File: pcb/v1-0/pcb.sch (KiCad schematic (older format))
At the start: 0 parts

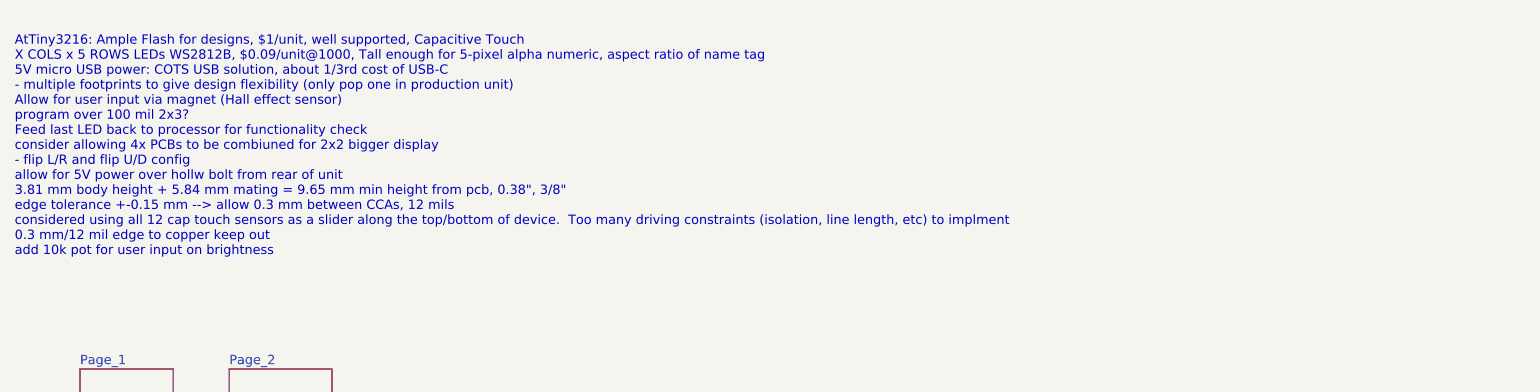
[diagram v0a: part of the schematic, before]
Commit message: compontnets placedr
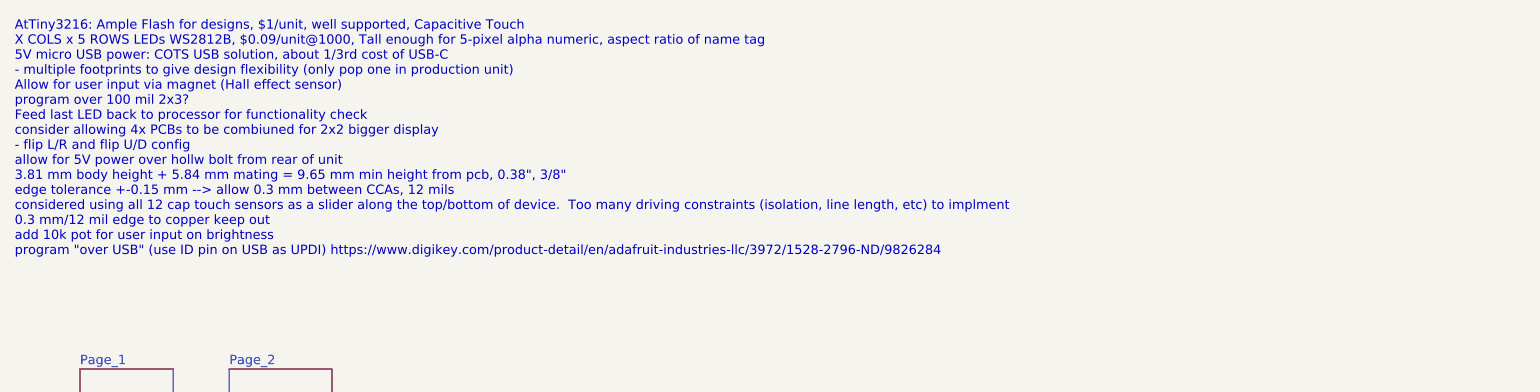
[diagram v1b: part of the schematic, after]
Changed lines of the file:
@@
 verify ws2182 footprint\nverify pinout of led\nwriteup parts list\nattiny: PTC, program, hall effect, USB power, Array led\n2x3 pin #s? conn_02x03\nallow for pogo programming\nensure LEDs are OFF during program upload\nadd UPDI pinout to silk screen\npick screw size, figure out PCB outline\nenter in space between traces into layout preferences\nbuy anodized aluminum\nbuy two color acrylic - info badge\nnameplate screws: threaded standoff caps\ndesign for enclosure - height from LEDs\ntwo-piece standoff panel-hanging brackets\ncaptive pins appear cheaper\nPlastic-Head Thumb Screws\n4-40, 0.33/screw: https://www.mcmaster.com/91185A233/\nusb port on reverse side? no - top side reflow only\nround corners of pcb\nput arrow on RxD and TxD showing data flow direciton\nSense Line thickness should be between 0.1mm to 0.5mm\n T: front panel thickness, 1.6 mm\n6" max line length on sense lines\nmcmaster: metal part to melt into plastic the rigidly hold screw - ref tail from hackaday
 Text Notes 550  1750 0    50   ~ 0
-AtTiny3216: Ample Flash for designs, $1/unit, well supported, Capacitive Touch\nX COLS x 5 ROWS LEDs WS2812B, $0.09/unit@1000, Tall enough for 5-pixel alpha numeric, aspect ratio of name tag\n5V micro USB power: COTS USB solution, about 1/3rd cost of USB-C\n- multiple footprints to give design flexibility (only pop one in production unit)\nAllow for user input via magnet (Hall effect sensor)\nprogram over 100 mil 2x3?\nFeed last LED back to processor for functionality check\nconsider allowing 4x PCBs to be combiuned for 2x2 bigger display\n- flip L/R and flip U/D config\nallow for 5V power over hollw bolt from rear of unit\n3.81 mm body height + 5.84 mm mating = 9.65 mm min height from pcb, 0.38", 3/8"\nedge tolerance +-0.15 mm --> allow 0.3 mm between CCAs, 12 mils\nconsidered using all 12 cap touch sensors as a slider along the top/bottom of device.  Too many driving constraints (isolation, line length, etc) to implment\n0.3 mm/12 mil edge to copper keep out\nadd 10k pot for user input on brightness
+AtTiny3216: Ample Flash for designs, $1/unit, well supported, Capacitive Touch\nX COLS x 5 ROWS LEDs WS2812B, $0.09/unit@1000, Tall enough for 5-pixel alpha numeric, aspect ratio of name tag\n5V micro USB power: COTS USB solution, about 1/3rd cost of USB-C\n- multiple footprints to give design flexibility (only pop one in production unit)\nAllow for user input via magnet (Hall effect sensor)\nprogram over 100 mil 2x3?\nFeed last LED back to processor for functionality check\nconsider allowing 4x PCBs to be combiuned for 2x2 bigger display\n- flip L/R and flip U/D config\nallow for 5V power over hollw bolt from rear of unit\n3.81 mm body height + 5.84 mm mating = 9.65 mm min height from pcb, 0.38", 3/8"\nedge tolerance +-0.15 mm --> allow 0.3 mm between CCAs, 12 mils\nconsidered using all 12 cap touch sensors as a slider along the top/bottom of device.  Too many driving constraints (isolation, line length, etc) to implment\n0.3 mm/12 mil edge to copper keep out\nadd 10k pot for user input on brightness\nprogram "over USB" (use ID pin on USB as UPDI) https://www.digikey.com/product-detail/en/adafruit-industries-llc/3972/1528-2796-ND/9826284
 $Sheet
 S 900  2350 500  150

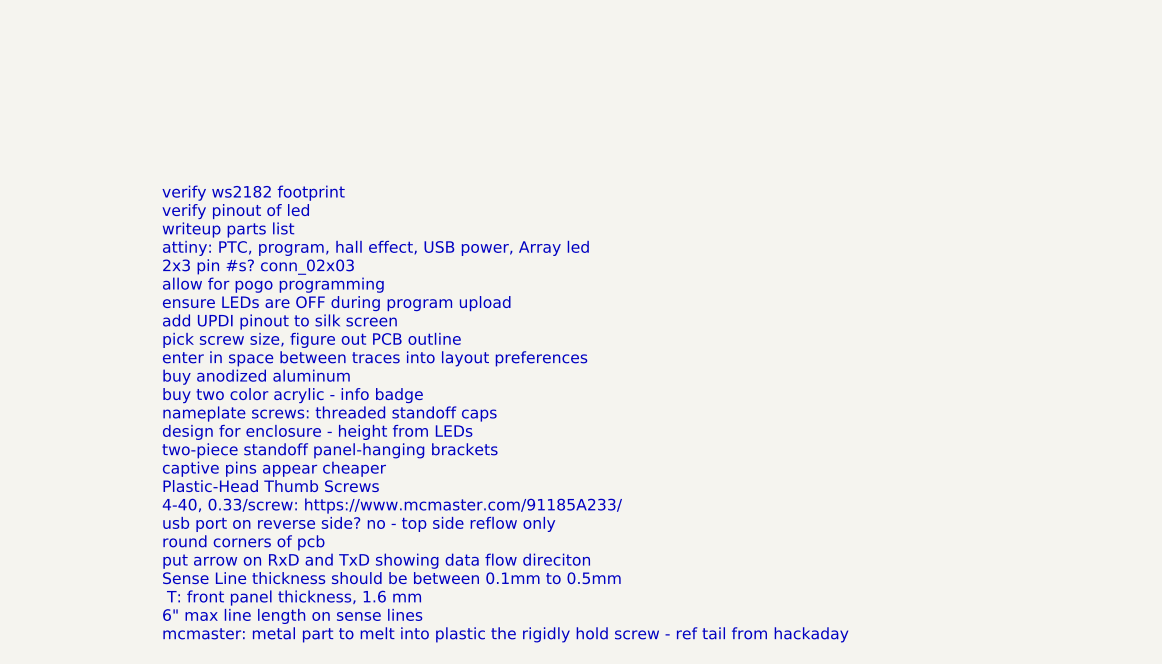
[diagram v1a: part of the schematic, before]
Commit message: candidate draft
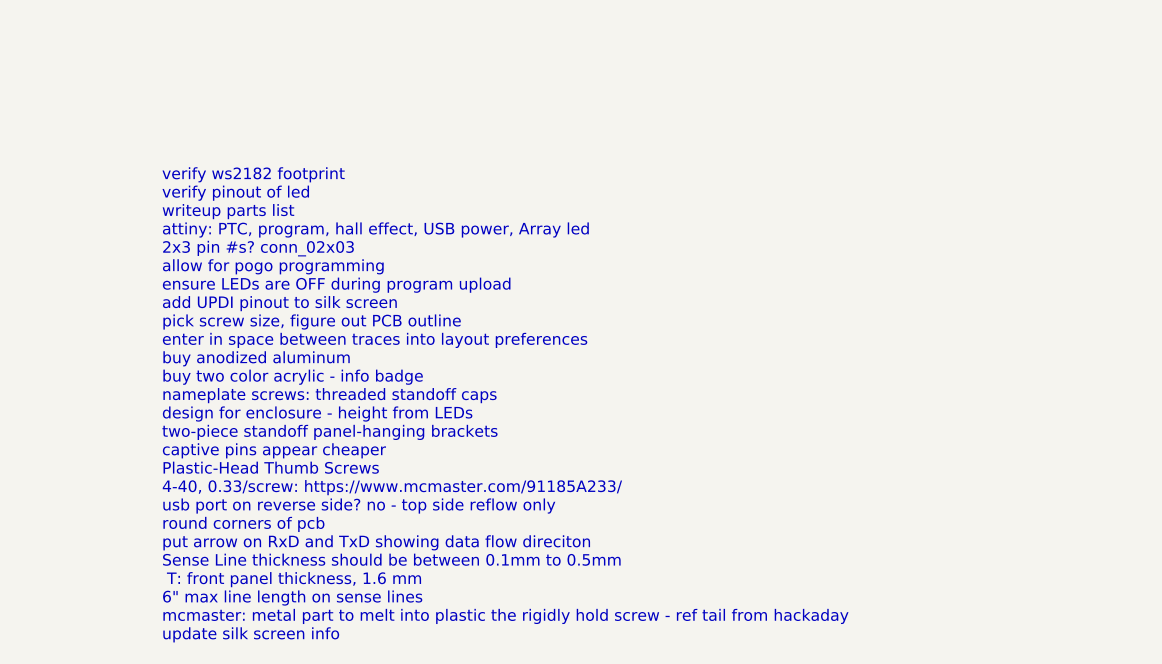
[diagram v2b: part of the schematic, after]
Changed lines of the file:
@@
 $EndDescr
 Text Notes 6950 6450 0    50   ~ 0
-verify ws2182 footprint\nverify pinout of led\nwriteup parts list\nattiny: PTC, program, hall effect, USB power, Array led\n2x3 pin #s? conn_02x03\nallow for pogo programming\nensure LEDs are OFF during program upload\nadd UPDI pinout to silk screen\npick screw size, figure out PCB outline\nenter in space between traces into layout preferences\nbuy anodized aluminum\nbuy two color acrylic - info badge\nnameplate screws: threaded standoff caps\ndesign for enclosure - height from LEDs\ntwo-piece standoff panel-hanging brackets\ncaptive pins appear cheaper\nPlastic-Head Thumb Screws\n4-40, 0.33/screw: https://www.mcmaster.com/91185A233/\nusb port on reverse side? no - top side reflow only\nround corners of pcb\nput arrow on RxD and TxD showing data flow direciton\nSense Line thickness should be between 0.1mm to 0.5mm\n T: front panel thickness, 1.6 mm\n6" max line length on sense lines\nmcmaster: metal part to melt into plastic the rigidly hold screw - ref tail from hackaday
+verify ws2182 footprint\nverify pinout of led\nwriteup parts list\nattiny: PTC, program, hall effect, USB power, Array led\n2x3 pin #s? conn_02x03\nallow for pogo programming\nensure LEDs are OFF during program upload\nadd UPDI pinout to silk screen\npick screw size, figure out PCB outline\nenter in space between traces into layout preferences\nbuy anodized aluminum\nbuy two color acrylic - info badge\nnameplate screws: threaded standoff caps\ndesign for enclosure - height from LEDs\ntwo-piece standoff panel-hanging brackets\ncaptive pins appear cheaper\nPlastic-Head Thumb Screws\n4-40, 0.33/screw: https://www.mcmaster.com/91185A233/\nusb port on reverse side? no - top side reflow only\nround corners of pcb\nput arrow on RxD and TxD showing data flow direciton\nSense Line thickness should be between 0.1mm to 0.5mm\n T: front panel thickness, 1.6 mm\n6" max line length on sense lines\nmcmaster: metal part to melt into plastic the rigidly hold screw - ref tail from hackaday\nupdate silk screen info
 Text Notes 550  1750 0    50   ~ 0
 AtTiny3216: Ample Flash for designs, $1/unit, well supported, Capacitive Touch\nX COLS x 5 ROWS LEDs WS2812B, $0.09/unit@1000, Tall enough for 5-pixel alpha numeric, aspect ratio of name tag\n5V micro USB power: COTS USB solution, about 1/3rd cost of USB-C\n- multiple footprints to give design flexibility (only pop one in production unit)\nAllow for user input via magnet (Hall effect sensor)\nprogram over 100 mil 2x3?\nFeed last LED back to processor for functionality check\nconsider allowing 4x PCBs to be combiuned for 2x2 bigger display\n- flip L/R and flip U/D config\nallow for 5V power over hollw bolt from rear of unit\n3.81 mm body height + 5.84 mm mating = 9.65 mm min height from pcb, 0.38", 3/8"\nedge tolerance +-0.15 mm --> allow 0.3 mm between CCAs, 12 mils\nconsidered using all 12 cap touch sensors as a slider along the top/bottom of device.  Too many driving constraints (isolation, line length, etc) to implment\n0.3 mm/12 mil edge to copper keep out\nadd 10k pot for user input on brightness\nprogram "over USB" (use ID pin on USB as UPDI) https://www.digikey.com/product-detail/en/adafruit-industries-llc/3972/1528-2796-ND/9826284
